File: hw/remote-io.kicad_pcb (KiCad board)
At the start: 2 copper layers, 65 x 56.5 mm, 63 parts, among them P1 CONN_01X02, P10 CONN_01X04, P11 CONN_01X02, P2 CONN_01X08, P3 CONN_01X08, P5 CONN_02X20, Q1 DMG2305UX, Q2 DMMT5401, U1 AP1506, U2 LP2992, U3 MCP3008, U4 CAT24C32, U6 MCP2515, U7 ADM3054, Y1 Crystal

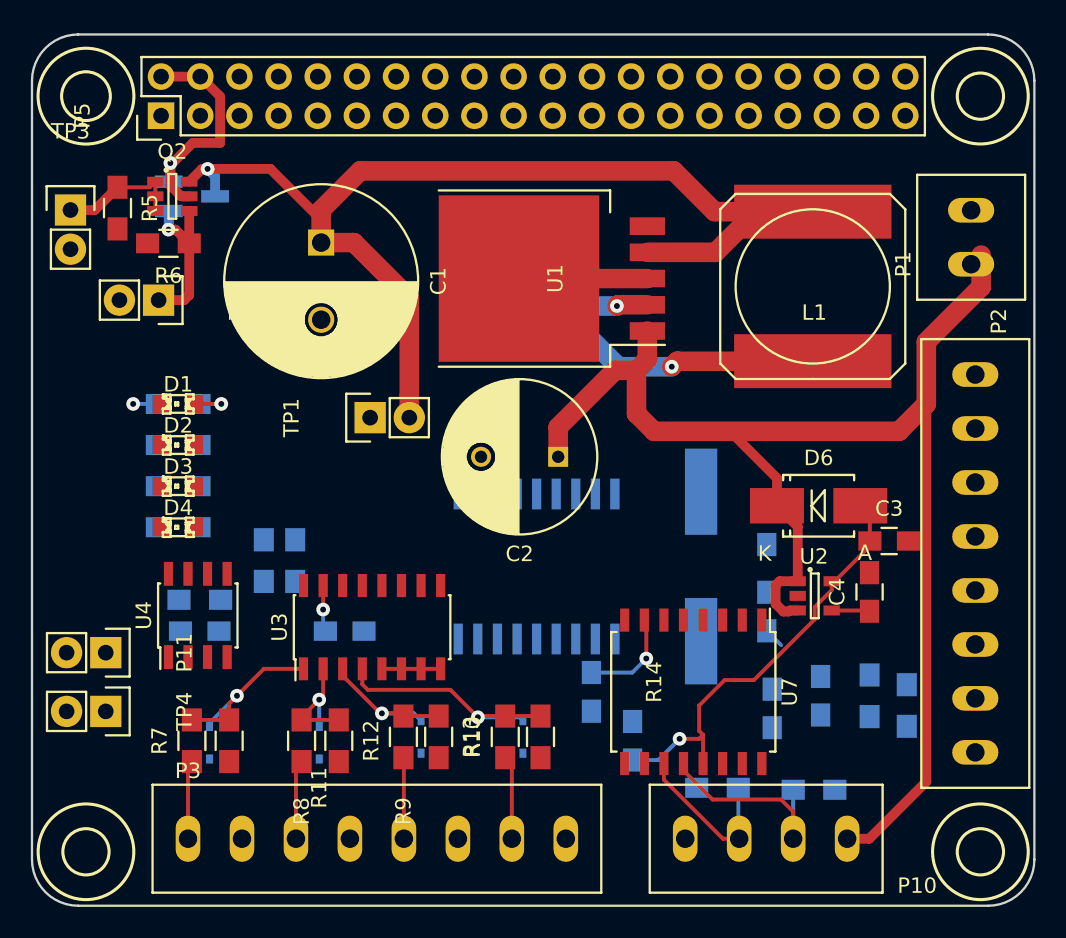
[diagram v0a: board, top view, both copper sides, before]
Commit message: Preliminary routing of board. Messy but whatever... it's a rev 0
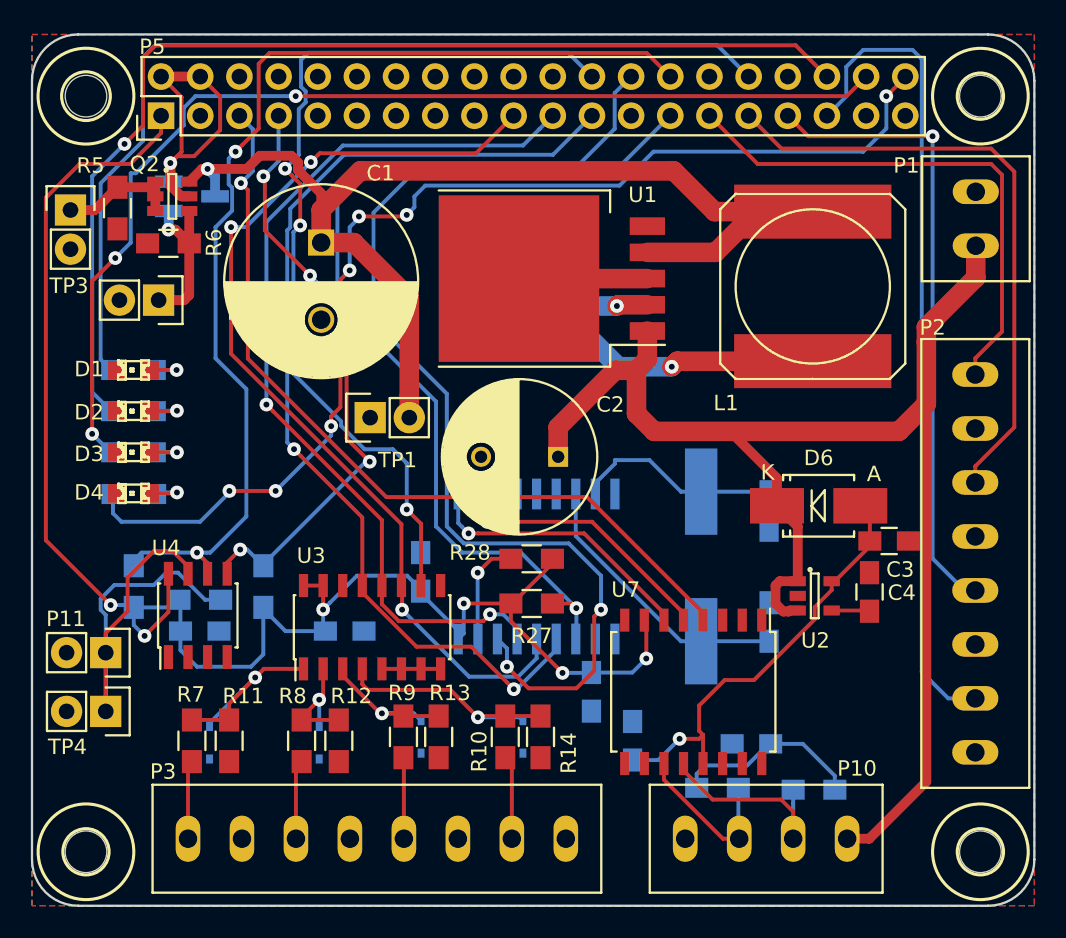
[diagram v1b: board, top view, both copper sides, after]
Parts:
- added REF**: MountingHole_2-7mm, Mounting_Holes:MountingHole_2-7mm, F.Cu at (90.5, 25.0)
- added REF**: MountingHole_2-7mm, Mounting_Holes:MountingHole_2-7mm, F.Cu at (90.5, 74.0)
- added REF**: MountingHole_2-7mm, Mounting_Holes:MountingHole_2-7mm, F.Cu at (32.5, 25.0)
- added REF**: MountingHole_2-7mm, Mounting_Holes:MountingHole_2-7mm, F.Cu at (32.5, 74.0)
- R27, R28: moved to F.Cu
- moved C12 27.2 mm to (54.2, 55.9)
- moved R27 25.2 mm to (61.4, 57.9), turned to 180 degrees
- moved R28 23.6 mm to (61.4, 55.0), turned to 0 degrees
- moved R23 8.60 mm to (35.6, 56.8)
- moved C10 6.52 mm to (76.8, 51.9), turned to 270 degrees
- moved C11 6.27 mm to (76.8, 59.1), turned to 90 degrees
- moved D2 3.64 mm to (35.6, 45.4)
- moved D3 3.64 mm to (35.6, 48.1)
- moved D4 3.64 mm to (35.6, 50.8)
- moved R2 3.64 mm to (35.6, 45.4)
- moved R3 3.64 mm to (35.6, 48.1)
- moved D1 3.64 mm to (35.6, 42.8)
- moved R1 3.64 mm to (35.6, 42.8)
- moved R4 3.60 mm to (35.6, 50.8)
- moved C13 2.67 mm to (75.7, 67.0), turned to 180 degrees
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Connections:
- U1 pad 3: Net-(U1-Pad3) -> GND
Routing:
- net +3V3: track 9.75 -> 107.3 mm, vias 2 -> 6
- net /CAN Controller and Transceiver/CAN_~CS: track 0.00 -> 74.3 mm, vias 0 -> 2
- net /LED3: track 0.00 -> 73.8 mm, vias 0 -> 7
- net /LED2: track 0.00 -> 70.7 mm, vias 0 -> 3
- net /LED1: track 0.00 -> 70.4 mm, vias 0 -> 1
- net /I2C ID EEPROM/ID_SC: track 0.00 -> 69.6 mm, vias 0 -> 2
- net /Battery Monitor/ADC_CLK: track 0.00 -> 66.0 mm, vias 0 -> 2
- net /Battery Monitor/ADC_DIN: track 0.00 -> 63.0 mm, vias 0 -> 3
- net /LED0: track 1.57 -> 62.2 mm, vias 1 -> 0
- net /Battery Monitor/ADC_DOUT: track 0.00 -> 59.8 mm, vias 0 -> 2
- net /Battery Monitor/ADC_~CS~/SHDN: track 0.19 -> 59.7 mm, vias 0 -> 3
- net /CAN Controller and Transceiver/CAN_VSENSE: track 0.00 -> 53.4 mm, vias 0 -> 1
- net /SW_IN3: track 0.00 -> 53.2 mm
- net /I2C ID EEPROM/ID_SD: track 0.00 -> 53.0 mm, vias 0 -> 3
- net /CAN Controller and Transceiver/CAN_~INT: track 0.00 -> 46.6 mm, vias 0 -> 3
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- added copper zone on B.Cu, net GND
- added copper zone on F.Cu, net GND
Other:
- net class Default: clearance 0.0254 -> 0.075
- rule trace_clearance: 0.0254 -> 0.075
